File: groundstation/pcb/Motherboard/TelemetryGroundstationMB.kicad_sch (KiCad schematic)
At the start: 105 parts, among them J1 USB-C, J2 USB-C, J3 ICD15S13E4GV00LF, J4 USB-C, J5 ICD15S13E4GV00LF, J6 ICD15S13E4GV00LF, J7 ICD15S13E4GV00LF, J8 Conn_01x06_Pin, M1 M4 Mounting Hole, M2 M4 Mounting Hole, M3 M4 Mounting Hole, M4 M4 Mounting Hole, Q1 NPN, U1 CP2102N, U2 CP2102N, U3 CP2102N, U4 MIC29300-5WU-TR, U5 AVR128DB64x-xPT, U6 MIC29300-3.3WU-TR

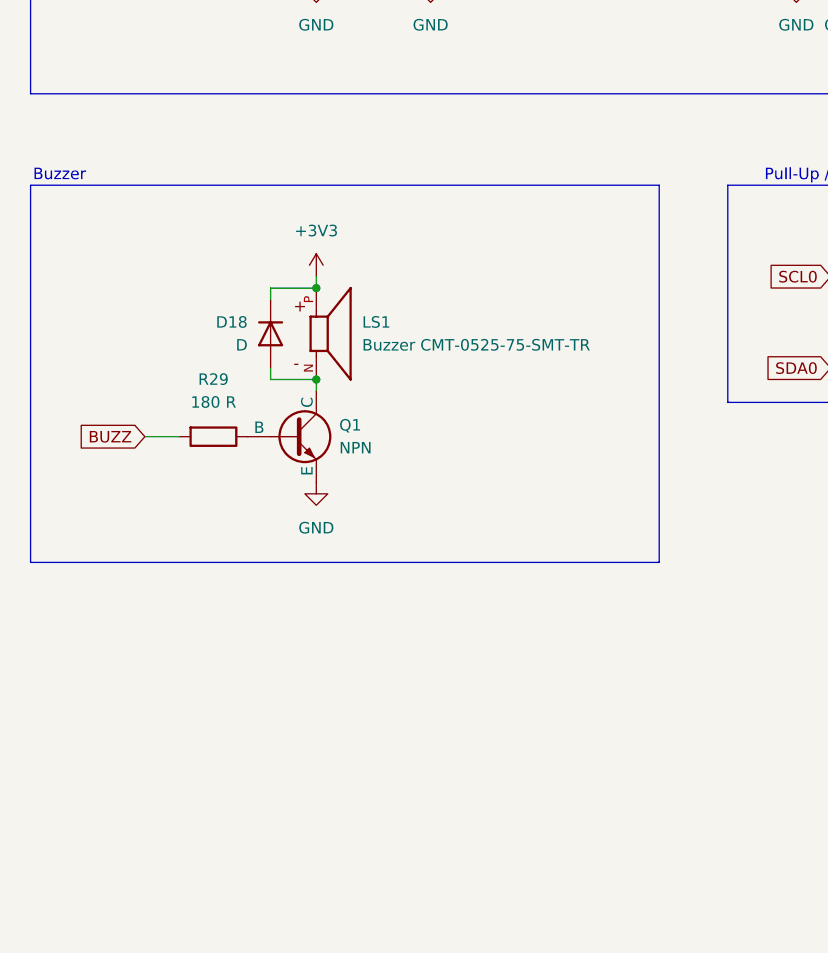
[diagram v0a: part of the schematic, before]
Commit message: update motherboard
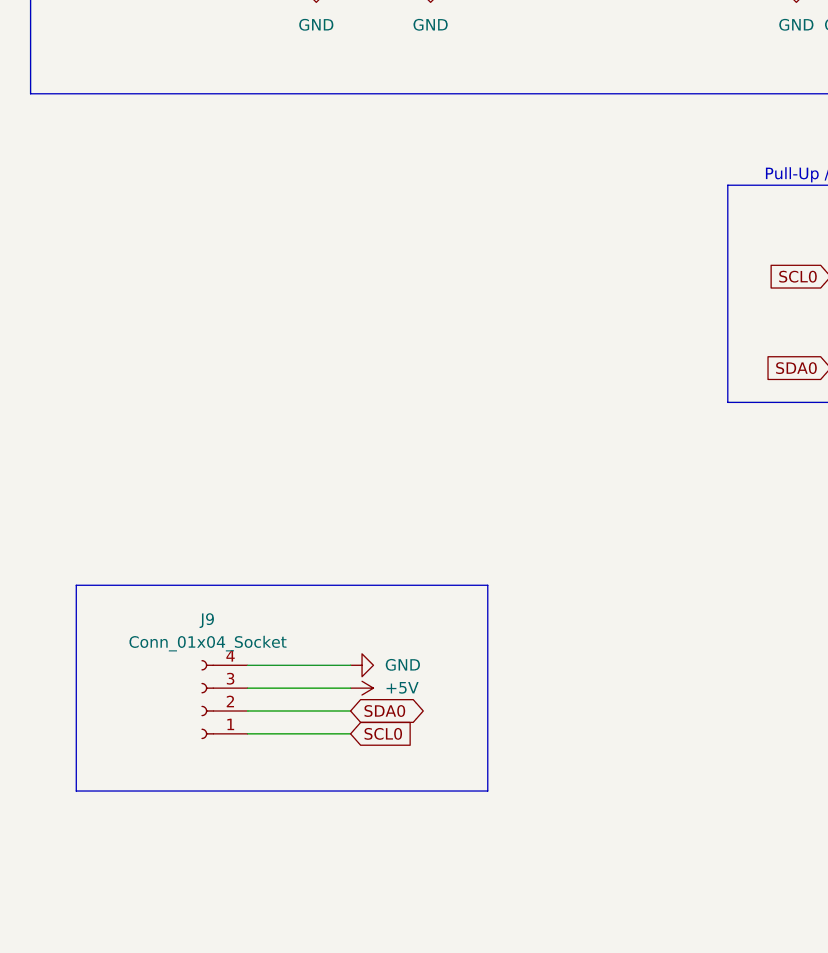
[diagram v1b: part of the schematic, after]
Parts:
- removed D18: D, Diode_SMD:D_SOD-123, symbol Device:D
- removed LS1: Buzzer CMT-0525-75-SMT-TR, Footprints:Buzzer XDCR_CMT-0525-75-SMT-TR, symbol Symbols:Buzzer CMT-0525-75-SMT-TR
- removed Q1: NPN, Package_TO_SOT_SMD:SOT-23, symbol Simulation_SPICE:NPN
- removed R29: 180 R, Resistor_SMD:R_0805_2012Metric_Pad1.20x1.40mm_HandSolder, symbol Device:R
- added J9: Conn_01x04_Socket, symbol Connector:Conn_01x04_Socket
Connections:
- net +5V: now also J9.3 (Pin_3)
- net GND: now also J9.4 (Pin_4)
- net SCL0: now also J9.1 (Pin_1)
- net SDA0: now also J9.2 (Pin_2)
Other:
- note removed: "Buzzer"
